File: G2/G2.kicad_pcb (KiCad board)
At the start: 2 copper layers, 156.2 x 187.5 mm, 242 parts, among them CON401 AVR-JTAG-10, J201 GS2, J202 GS2, J301 GS3, J302 GS3, J303 GS3, J304 GS3, J305 GS3, J306 GS3, J307 GS3, J308 GS3, J309 Conn_02x08_Odd_Even, J310 Conn_02x08_Odd_Even, J311 Conn_01x09, J312 Conn_01x09, J313 Conn_01x09, J314 Conn_01x09, J315 Conn_01x09, J316 Conn_01x09, J401 Conn_01x07, J402 Conn_02x08_Odd_Even, J403 Conn_02x04_Counter_Clockwise, J601 Conn_02x08_Odd_Even, Q301 ZXTN25050DFHTA, Q302 ZXTN25050DFHTA, Q303 ZXTN25050DFHTA, Q304 ZXTN25050DFHTA, Q305 ZXTN25050DFHTA, Q306 ZXTN25050DFHTA, Q307 ZXTN25050DFHTA, Q308 ZXTN25050DFHTA, Q309 ZXTN25050DFHTA, Q310 ZXTN25050DFHTA, U201 LM1084-3.3, U202 LM1084-5.0, U301 LTV-354T, U302 LTV-354T, U303 LTV-354T, U304 LTV-354T, U305 LTV-354T, U306 LTV-354T, U307 LTV-354T, U308 LTV-354T, U309 MCP23017, U401 TXB0102DCU, U501 ADS1115IDGST, U502 ADS1115IDGST, U601 TXB0102DCU

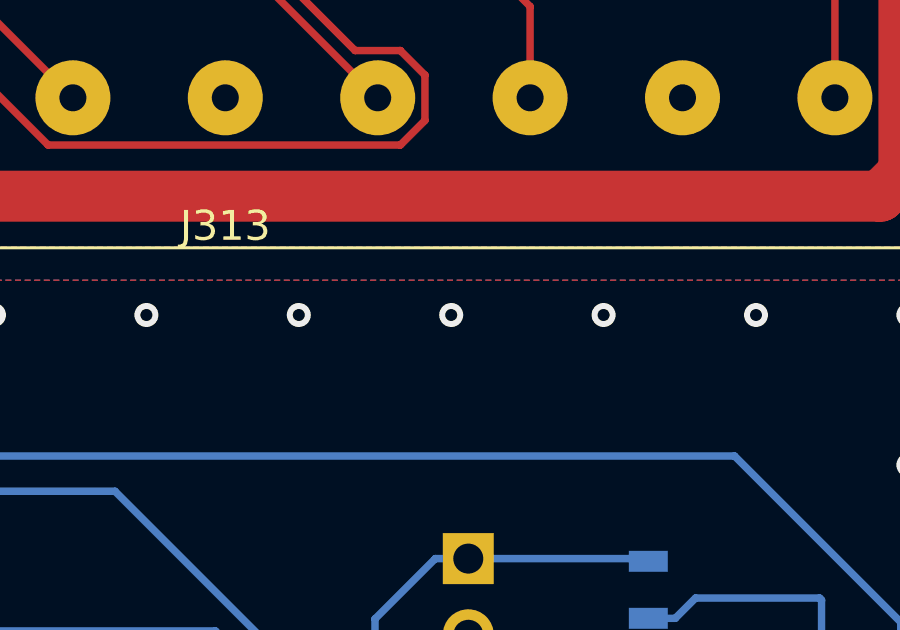
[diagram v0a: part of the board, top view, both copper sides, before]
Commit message: Fixed a via issue
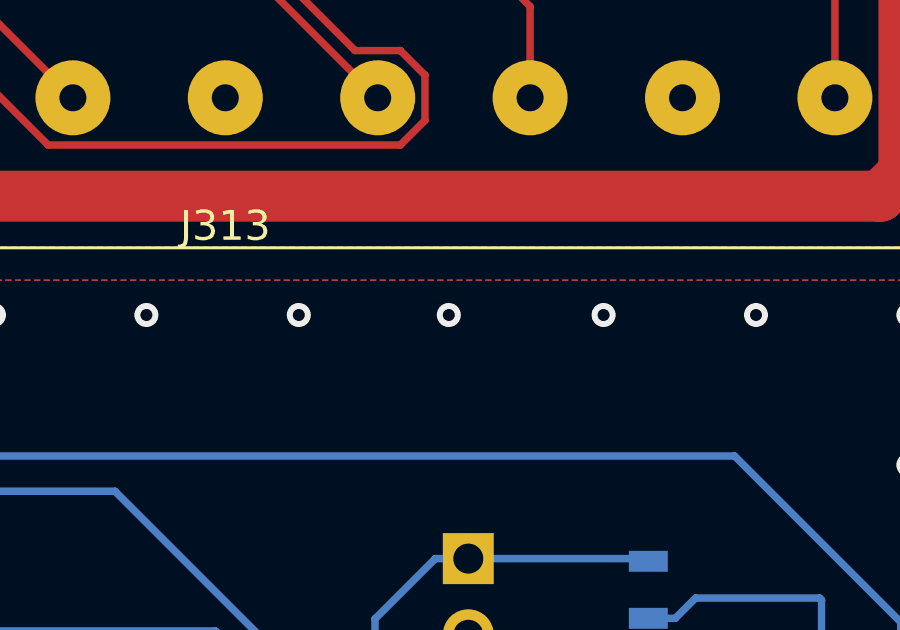
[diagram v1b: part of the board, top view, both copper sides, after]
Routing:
- net GND_C: vias 92 -> 93
- net (no net): vias 1 -> 0
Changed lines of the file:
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@@
     (pcbplotparams
       (layerselection 0x011f0_ffffffff)
-      (usegerberextensions true)
+      (usegerberextensions false)
       (usegerberattributes true)
       (usegerberadvancedattributes true)
@@
   (segment (start 152.57 118.86) (end 152.57 120.11) (width 0.25) (layer F.Cu) (net 29))
   (segment (start 152.57 120.11) (end 152.57 141.72) (width 0.25) (layer F.Cu) (net 29))
+  (via (at 150.75 100.87) (size 0.8) (drill 0.4) (layers F.Cu B.Cu) (net 187))
   (via (at 93.5 118.68) (size 0.8) (drill 0.4) (layers F.Cu B.Cu) (net 187))
   (via (at 88.36 118.72) (size 0.8) (drill 0.4) (layers F.Cu B.Cu) (net 187))
@@
   (via (at 160.99 100.87) (size 0.8) (drill 0.4) (layers F.Cu B.Cu) (net 187))
   (via (at 155.91 100.87) (size 0.8) (drill 0.4) (layers F.Cu B.Cu) (net 187))
-  (via (at 150.83 100.87) (size 0.8) (drill 0.4) (layers F.Cu B.Cu) (net 0))
   (via (at 145.75 100.87) (size 0.8) (drill 0.4) (layers F.Cu B.Cu) (net 187))
   (via (at 140.67 100.87) (size 0.8) (drill 0.4) (layers F.Cu B.Cu) (net 187))
